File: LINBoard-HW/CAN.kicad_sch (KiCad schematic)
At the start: 11 parts, among them U6 MCP25625x-x-ML, Y2 16MHz 12pF

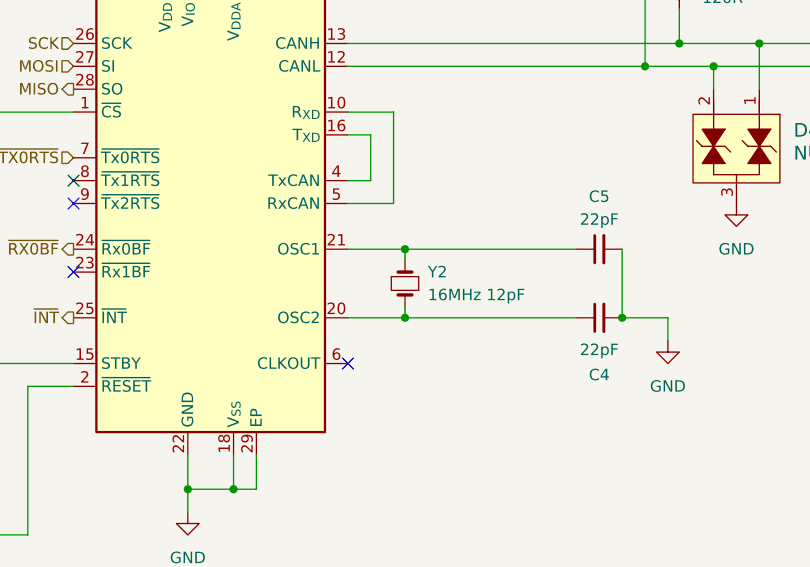
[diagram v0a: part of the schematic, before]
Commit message: board layout started
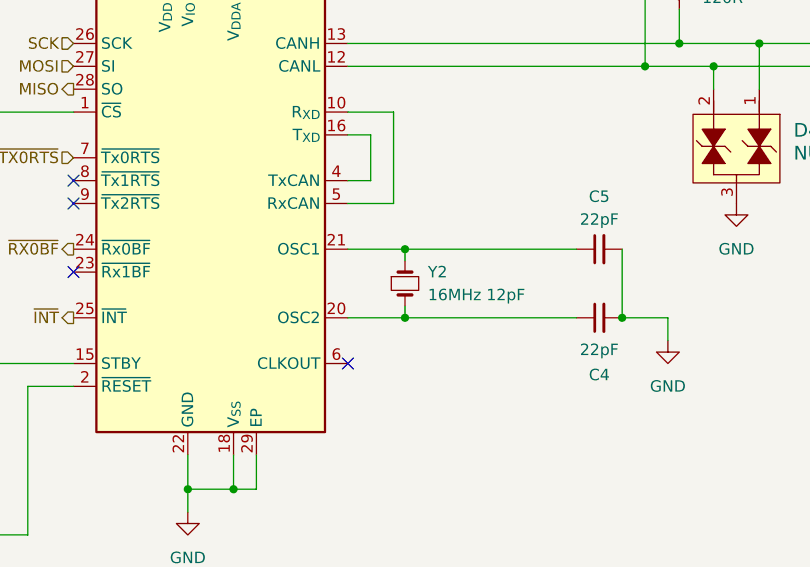
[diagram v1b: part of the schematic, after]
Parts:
- C3, C4, C5: footprint Capacitor_SMD:C_0603_1608Metric -> Capacitor_SMD:C_0402_1005Metric
- R17, R18, R19, R4: footprint Resistor_SMD:R_0603_1608Metric -> Resistor_SMD:R_0402_1005Metric
- Y2: footprint (none) -> Crystal:Crystal_SMD_3225-4Pin_3.2x2.5mm
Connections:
- net at C4.1, U6.20 (OSC2): now also Y2.2; no longer Y2.1
- net at C5.1, U6.21 (OSC1): now also Y2.1; no longer Y2.2
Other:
- moved on the sheet: Y2
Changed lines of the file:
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@@
 			)
 		)
-		(property "Footprint" "Resistor_SMD:R_0603_1608Metric"
+		(property "Footprint" "Resistor_SMD:R_0402_1005Metric"
 			(at 102.87 137.16 0)
 			(effects
@@
 			)
 		)
-		(property "Footprint" "Resistor_SMD:R_0603_1608Metric"
+		(property "Footprint" "Resistor_SMD:R_0402_1005Metric"
 			(at 102.87 118.11 0)
 			(effects
@@
 			)
 		)
-		(property "Footprint" "Capacitor_SMD:C_0603_1608Metric"
+		(property "Footprint" "Capacitor_SMD:C_0402_1005Metric"
 			(at 172.72 105.41 0)
 			(effects
@@
 			)
 		)
-		(property "Footprint" "Capacitor_SMD:C_0603_1608Metric"
+		(property "Footprint" "Capacitor_SMD:C_0402_1005Metric"
 			(at 172.72 113.03 0)
 			(effects
@@
 	(symbol
 		(lib_id "Device:Crystal_Small")
-		(at 151.13 109.22 90)
+		(at 151.13 109.22 270)
 		(unit 1)
 		(exclude_from_sim no)
@@
 					(size 1.27 1.27)
 				)
-				(justify right)
+				(justify left)
 			)
 		)
@@
 					(size 1.27 1.27)
 				)
-				(justify right)
-			)
-		)
-		(property "Footprint" ""
+				(justify left)
+			)
+		)
+		(property "Footprint" "Crystal:Crystal_SMD_3225-4Pin_3.2x2.5mm"
 			(at 151.13 109.22 0)
 			(effects
@@
 			)
 		)
-		(property "Footprint" "Resistor_SMD:R_0603_1608Metric"
+		(property "Footprint" "Resistor_SMD:R_0402_1005Metric"
 			(at 102.87 90.17 0)
 			(effects
@@
 			)
 		)
-		(property "Footprint" "Resistor_SMD:R_0603_1608Metric"
+		(property "Footprint" "Resistor_SMD:R_0402_1005Metric"
 			(at 181.61 76.2 0)
 			(effects
@@
 			)
 		)
-		(property "Footprint" "Capacitor_SMD:C_0603_1608Metric"
+		(property "Footprint" "Capacitor_SMD:C_0402_1005Metric"
 			(at 207.01 46.99 0)
 			(effects
